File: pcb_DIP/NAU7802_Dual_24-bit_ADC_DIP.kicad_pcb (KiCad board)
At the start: 2 copper layers, 50.8 x 22.9 mm, 35 parts, among them J1 CELL_A, J2 CELL_B, J3 STEMMA_QT, J4 STEMMA_QT, M1 Feather_M4_Express, U1 NAU7802

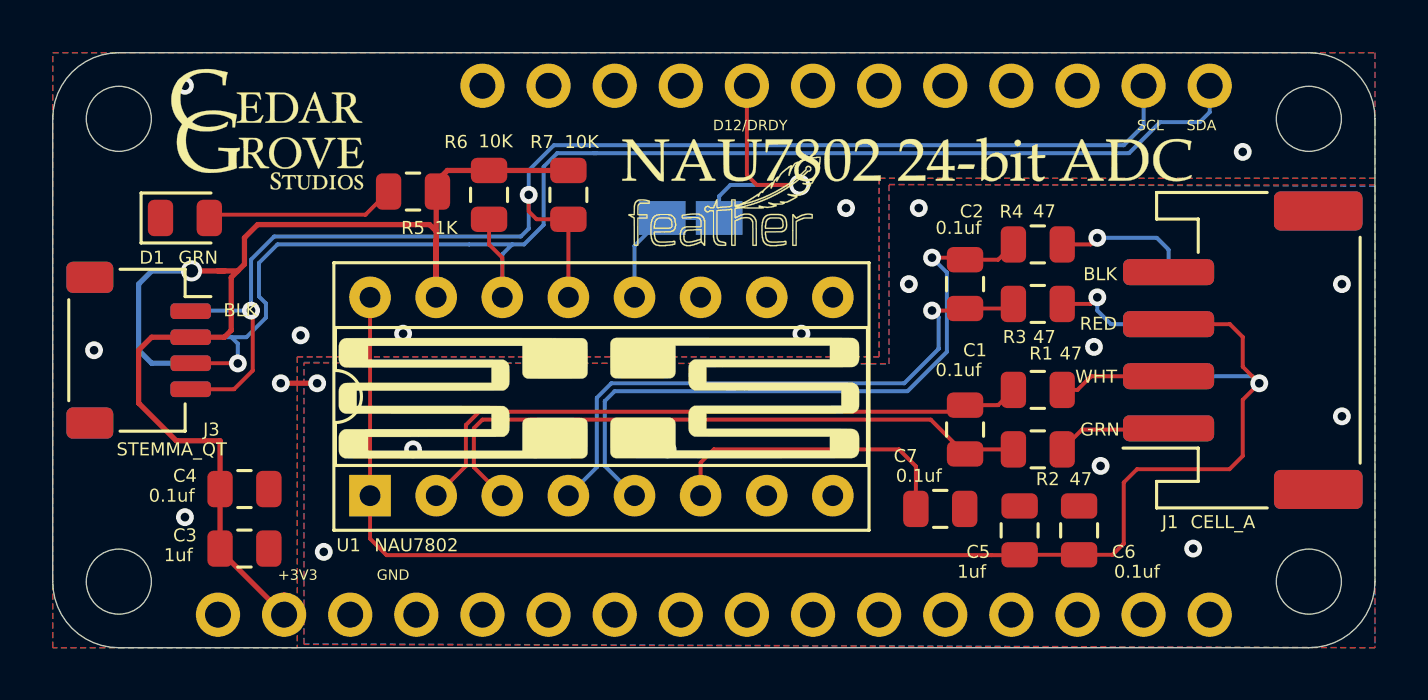
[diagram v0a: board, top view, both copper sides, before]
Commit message: update to newest kicad version
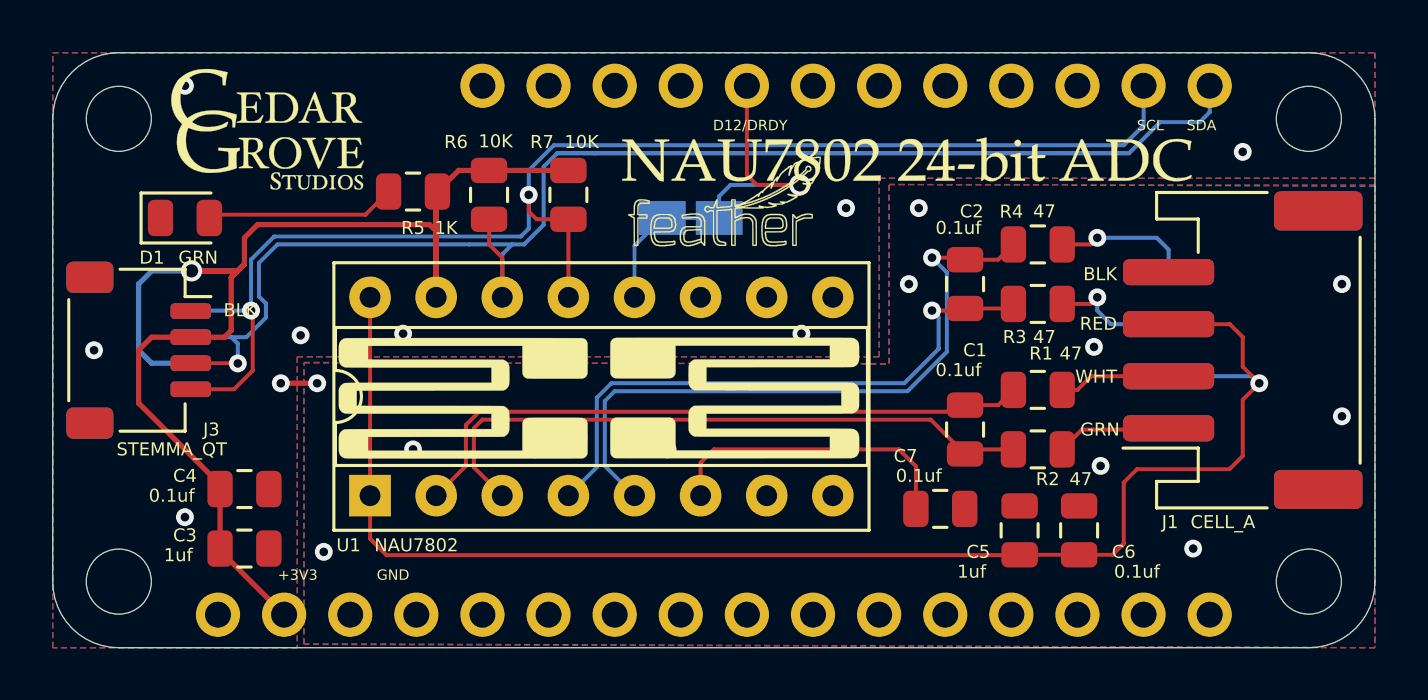
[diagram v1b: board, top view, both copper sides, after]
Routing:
- net /SDA: track 55.1 -> 77.1 mm
- net +3V3: track 50.7 -> 55.1 mm
- net /DRDY: track 16.0 -> 15.4 mm
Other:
- net class Default removed
- net class Power removed
